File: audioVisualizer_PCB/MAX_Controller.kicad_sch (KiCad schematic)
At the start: 16 parts, among them J10 Conn_01x08_Socket, J11 Conn_01x08_Socket, J12 Conn_01x08_Socket, J5 Conn_01x08_Socket, J6 Conn_01x08_Socket, J7 Conn_01x08_Socket, J8 Conn_01x08_Socket, J9 Conn_01x08_Socket, U3 MAX7219, U4 MAX7219, U5 MAX7219, U6 MAX7219

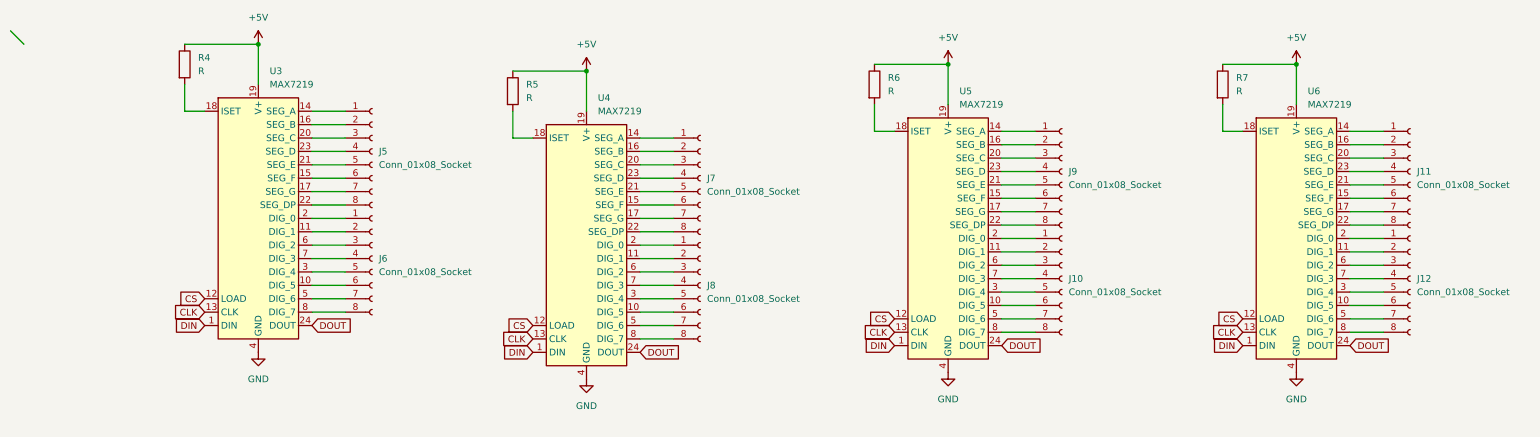
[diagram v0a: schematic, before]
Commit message: embeddeding the mcu is harder than I thought
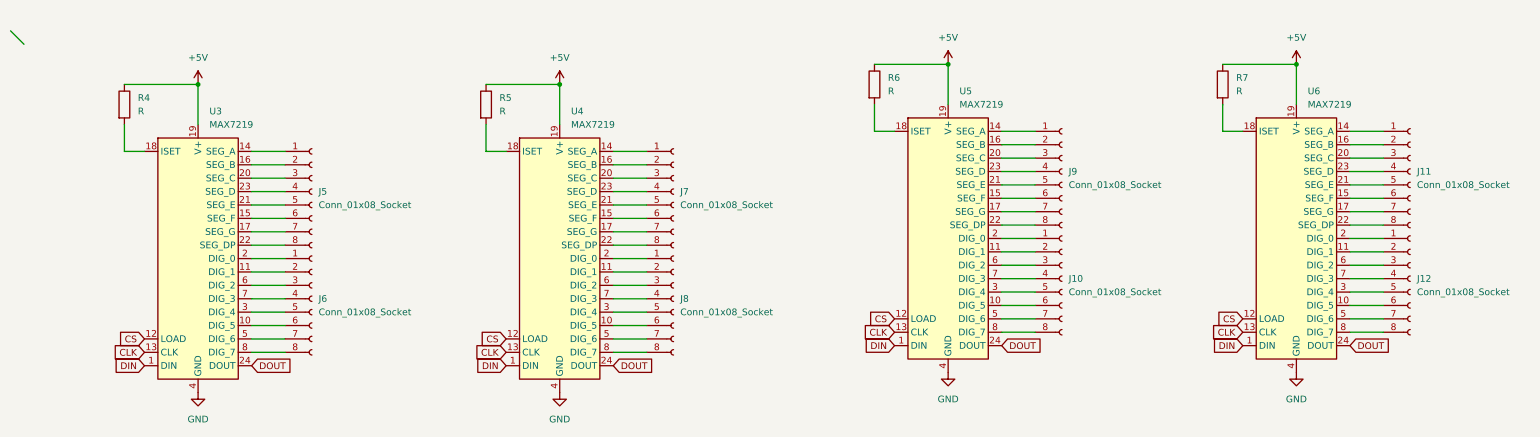
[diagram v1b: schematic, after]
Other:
- moved on the sheet: J5, J6, J7, J8, R4, R5, U3, U4
